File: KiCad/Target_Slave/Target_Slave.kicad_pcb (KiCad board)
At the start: 2 copper layers, 76.2 x 50.8 mm, 44 parts, among them J1 ICSP, J2 I2C, J3 I2C, SW1 I2C Address, U1 PIC16F1788-IP, U2 TSSP4038, U3 TSOP53456

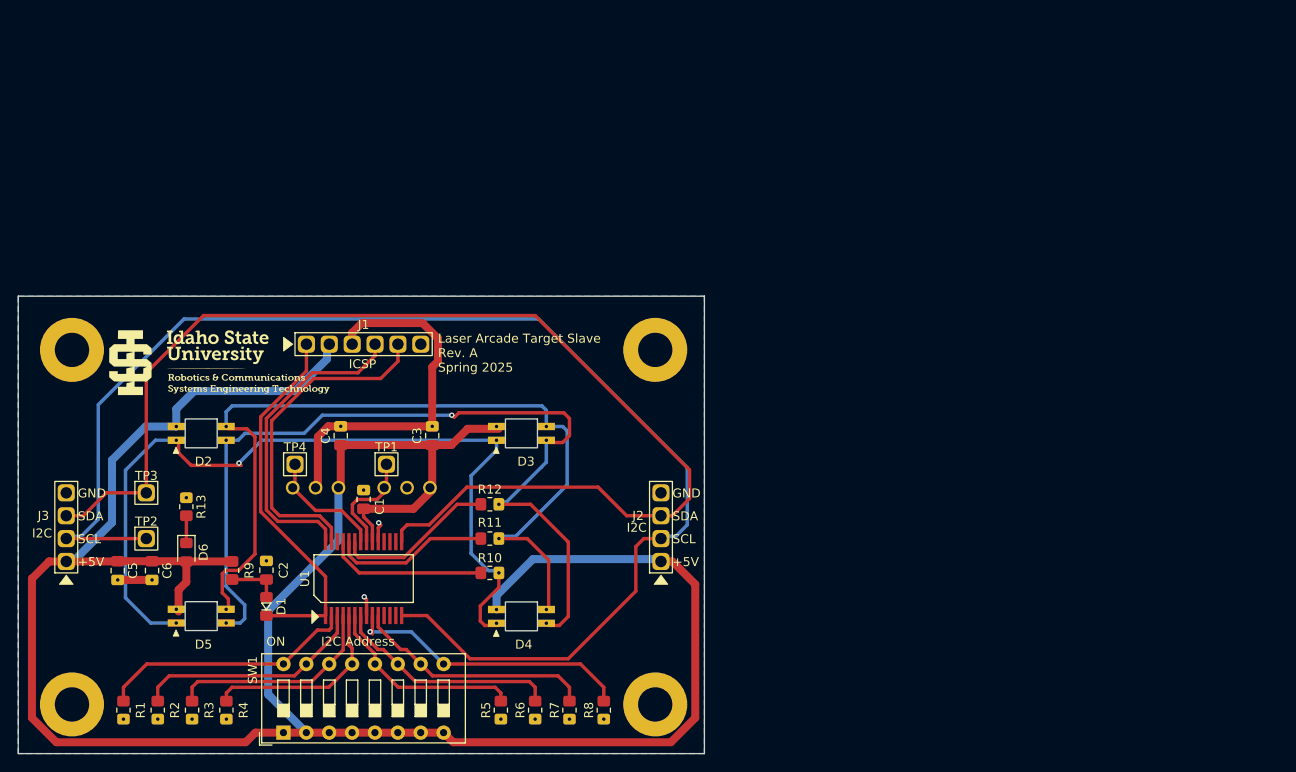
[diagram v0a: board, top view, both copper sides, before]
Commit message: Rev B Target Slave PCB design
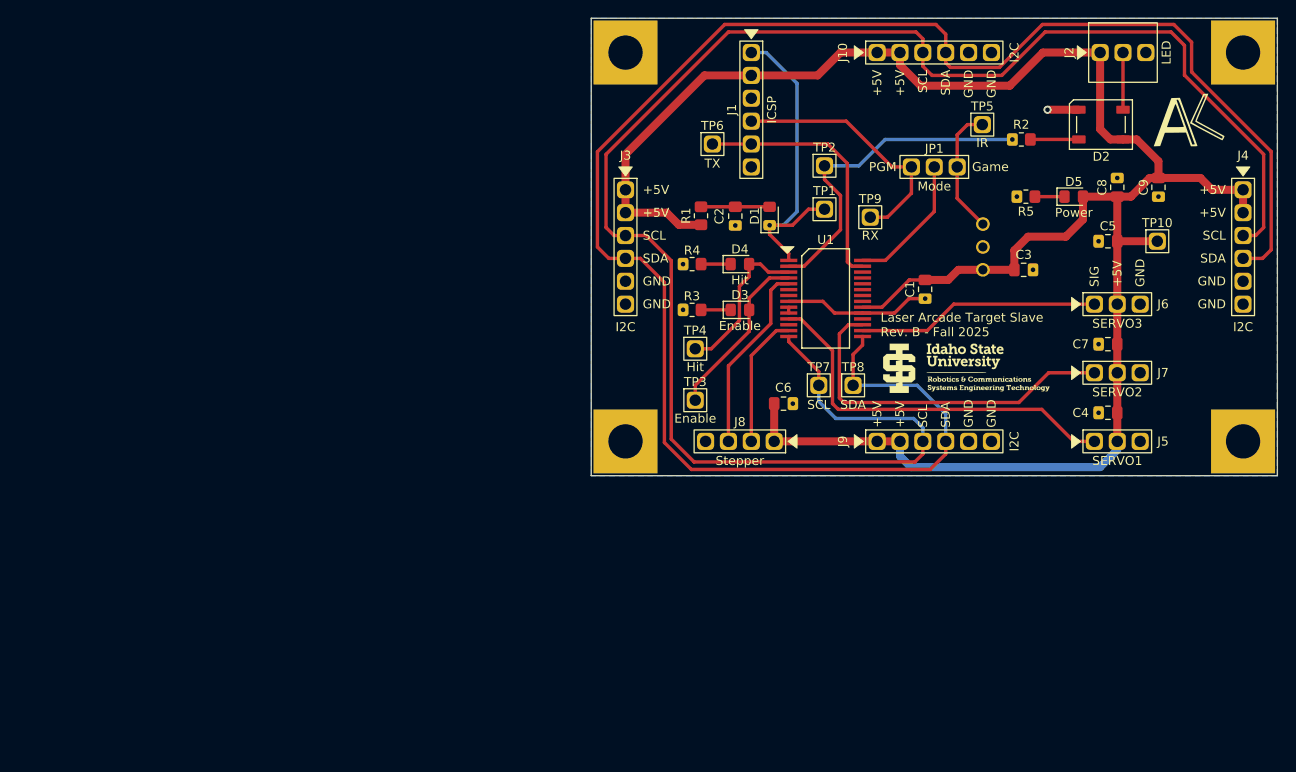
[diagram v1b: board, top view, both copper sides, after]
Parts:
- removed ? (x3): , 
- removed D6: LED, LED_SMD:LED_0805_2012Metric_Pad1.15x1.40mm_HandSolder
- removed the G*** at (135.4, 83.2)
- removed the G*** at (132.0, 118.1)
- removed the G*** at (121.2, 112.8)
- removed R10, R12: 90Ω, Resistor_SMD:R_0805_2012Metric_Pad1.20x1.40mm_HandSolder
- removed R11: 150Ω, Resistor_SMD:R_0805_2012Metric_Pad1.20x1.40mm_HandSolder
- removed R13: 4.7kΩ, Resistor_SMD:R_0805_2012Metric_Pad1.20x1.40mm_HandSolder
- removed R6, R7, R8: 330Ω, Resistor_SMD:R_0805_2012Metric_Pad1.20x1.40mm_HandSolder
- removed R9: 10kΩ, Resistor_SMD:R_0805_2012Metric_Pad1.20x1.40mm_HandSolder
- removed the REF** at (183.6, 81.9)
- removed SW1: I2C Address, 0_AKeller_Footprints:SW_DIP_SPSTx08_Slide_9.78x22.5mm_W7.62mm_P2.54mm
- removed U3: TSOP53456, 0_AKeller_Footprints:IR Receiver
- added C7: 1µF, Capacitor_SMD:C_0805_2012Metric_Pad1.18x1.45mm_HandSolder, F.Cu at (233.9, 81.3)
- added C8: 22uF, Capacitor_SMD:C_0805_2012Metric_Pad1.18x1.45mm_HandSolder, F.Cu at (234.9, 63.9)
- added C9: 0.1uF, Capacitor_SMD:C_0805_2012Metric_Pad1.18x1.45mm_HandSolder, F.Cu at (239.5, 63.9)
- added G***: LOGO, 2025 Logos:AKeller_Logo_0-23x0-31, F.Cu at (243.0, 56.4)
- added G***: LOGO, 2025 Logos:RCET Stacked 0-25x0_76, F.Cu at (218.3, 83.8)
- added J10: I2C, 0_AKeller_Footprints:1x6_100mil_Header, F.Cu at (214.6, 48.9)
- added J4: I2C, 0_AKeller_Footprints:1x6_100mil_Header, F.Cu at (248.9, 70.5)
- added J5: SERVO1, 0_AKeller_Footprints:1x3_100mil_Header, F.Cu at (234.9, 92.1)
- added J6: SERVO3, 0_AKeller_Footprints:1x3_100mil_Header, F.Cu at (234.9, 76.8)
- added J7: SERVO2, 0_AKeller_Footprints:1x3_100mil_Header, F.Cu at (234.9, 84.5)
- added J8: Stepper, 0_AKeller_Footprints:1x4_100mil_Header, F.Cu at (193.0, 92.1)
- added J9: I2C, 0_AKeller_Footprints:1x6_100mil_Header, F.Cu at (214.6, 92.1)
- added JP1: Mode, 0_AKeller_Footprints:1x3_100mil_Jumper, F.Cu at (214.6, 61.6)
- added REF**: M3 Mounting, 0_AKeller_Footprints:M3 Mounting, F.Cu at (180.3, 92.1)
- added REF**: M3 Mounting, 0_AKeller_Footprints:M3 Mounting, F.Cu at (248.9, 92.1)
- added REF**: M3 Mounting, 0_AKeller_Footprints:M3 Mounting, F.Cu at (180.3, 48.9)
- added REF**: M3 Mounting, 0_AKeller_Footprints:M3 Mounting, F.Cu at (248.9, 48.9)
- added TP10: PWR, 0_AKeller_Footprints:1x1_100mil_Header, F.Cu at (239.4, 69.8)
- added TP5: IR, 0_AKeller_Footprints:1x1_100mil_Header, F.Cu at (220.0, 56.9)
- added TP6: TX, 0_AKeller_Footprints:1x1_100mil_Header, F.Cu at (190.0, 59.1)
- added TP7: SCL, 0_AKeller_Footprints:1x1_100mil_Header, F.Cu at (201.8, 85.9)
- added TP8: SDA, 0_AKeller_Footprints:1x1_100mil_Header, F.Cu at (205.6, 85.9)
- added TP9: RX, 0_AKeller_Footprints:1x1_100mil_Header, F.Cu at (207.5, 67.2)
- C4: value 1uF -> 1µF
- C5: value 22uF -> 1µF
- C6: value 0.1uF -> 1µF
- D1: footprint 0_AKeller_Footprints:Diode_0805 -> Diode_SMD:D_0805_2012Metric_Pad1.15x1.40mm_HandSolder
- D2: value IN-P32TRRRGB -> WS2812B; footprint 0_AKeller_Footprints:IN-P32TRRRGB -> LED_SMD:LED_WS2812B_PLCC4_5.0x5.0mm_P3.2mm; moved to F.Cu
- D3: value IN-P32TRRRGB -> Enable; footprint 0_AKeller_Footprints:IN-P32TRRRGB -> LED_SMD:LED_0805_2012Metric_Pad1.15x1.40mm_HandSolder; moved to F.Cu
- D4: value IN-P32TRRRGB -> Hit; footprint 0_AKeller_Footprints:IN-P32TRRRGB -> LED_SMD:LED_0805_2012Metric_Pad1.15x1.40mm_HandSolder; moved to F.Cu
- D5: value IN-P32TRRRGB -> Power; footprint 0_AKeller_Footprints:IN-P32TRRRGB -> LED_SMD:LED_0805_2012Metric_Pad1.15x1.40mm_HandSolder; moved to F.Cu
- J2: value I2C -> LED; footprint 0_AKeller_Footprints:1x4_100mil_Header -> 0_AKeller_Footprints:1x3_100mil_Header_Locking
- J3: footprint 0_AKeller_Footprints:1x4_100mil_Header -> 0_AKeller_Footprints:1x6_100mil_Header
- R1: value 330Ω -> 10kΩ
- R2: value 330Ω -> 470Ω
- R3, R4, R5: value 330Ω -> 4.7kΩ
- TP1: value ~ -> MCLR
- TP2: value ~ -> RGB_IN
- TP3: value ~ -> Enable
- TP4: value ~ -> Hit
- moved C5 115.9 mm to (233.9, 69.8), turned to 0 degrees
- moved R2 114.9 mm to (224.3, 58.5), turned to 0 degrees
- moved D5 107.5 mm to (230.1, 64.9), turned to 0 degrees
- moved D2 105.6 mm to (233.1, 56.9)
- moved TP2 85.9 mm to (202.4, 61.5)
- moved C4 85.2 mm to (233.9, 88.9), turned to 0 degrees
- moved R1 84.4 mm to (188.7, 67.0)
- moved R5 81.6 mm to (224.8, 64.9), turned to 180 degrees
- moved J2 73.6 mm to (235.6, 48.9), turned to 0 degrees
- moved C6 72.5 mm to (197.9, 87.9), turned to 180 degrees
- moved R4 71.6 mm to (187.7, 72.4), turned to 180 degrees
- moved R3 71.1 mm to (187.7, 77.5), turned to 180 degrees
- moved D1 70.7 mm to (196.3, 67.0)
- moved J3 69.5 mm to (180.3, 70.5), turned to -90 degrees
- moved U2 69.3 mm to (220.0, 70.5), turned to -90 degrees
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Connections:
- net RB6 renamed TX
- C4 pad 1: +5V -> GND
- C4 pad 2: GND -> +5V
- C5 pad 1: +5V -> GND
- C5 pad 2: GND -> +5V
- C6 pad 1: +5V -> GND
- C6 pad 2: GND -> +5V
- D1 pad 1: Net-(D1-K) -> /MCLR
- D2 pad 1: Net-(D2-BK) -> +5V
- D2 pad 2: Net-(D2-GK) -> Net-(D2-DOUT)
- D2 pad 3: Net-(D2-RK) -> GND
- D2 pad 4: +5V -> Net-(D2-DIN)
- D3 pad 1: Net-(D2-BK) -> Net-(D3-K)
- D3 pad 2: Net-(D2-GK) -> Net-(D3-A)
- D4 pad 1: Net-(D2-BK) -> Net-(D4-K)
- D4 pad 2: Net-(D2-GK) -> Net-(D4-A)
- D5 pad 1: Net-(D2-BK) -> Net-(D5-K)
- D5 pad 2: Net-(D2-GK) -> +5V
- J1 pad 1: Net-(D1-K) -> /MCLR
- J1 pad 4: RB7 -> RX
- J2 pad 2: Net-(U1-RC3/SCK/SCL) -> Net-(D2-DOUT)
- J2 pad 3: Net-(U1-RC4/SDI/SDA) -> GND
- J3 pad 2: Net-(U1-RC3/SCK/SCL) -> +5V
- J3 pad 3: Net-(U1-RC4/SDI/SDA) -> /SCL
- J3 pad 4: GND -> /SDA
- R1 pad 1: GND -> +5V
- R1 pad 2: /RA0 -> Net-(D1-A)
- R2 pad 1: GND -> Net-(U1-ULPWU/C12IN0-/AN0/RA0)
- R2 pad 2: /RA1 -> Net-(D2-DIN)
- R3 pad 1: GND -> Net-(D3-K)
- R3 pad 2: /RA2 -> GND
- R4 pad 1: GND -> Net-(D4-K)
- R4 pad 2: /RA3 -> GND
- R5 pad 1: GND -> Net-(D5-K)
- R5 pad 2: /RA4 -> GND
- TP1 pad 1: Net-(U1-INT/AN12/RB0) -> /MCLR
- TP2 pad 1: Net-(U1-RC3/SCK/SCL) -> Net-(U1-ULPWU/C12IN0-/AN0/RA0)
- TP3 pad 1: Net-(U1-RC4/SDI/SDA) -> Net-(D3-A)
- TP4 pad 1: Net-(U1-P1C/AN10/RB1) -> Net-(D4-A)
- U1 pad 1: Net-(D1-K) -> /MCLR
- U1 pad 10: /RA6 -> Net-(U1-CLKIN/OSC1/RA7)
- U1 pad 11: unconnected-(U1-RC0/T1OSO/T1CK1-Pad11) -> SERVO1
- U1 pad 13: unconnected-(U1-RC2/P1A/CCP1-Pad13) -> STEP
- U1 pad 14: Net-(U1-RC3/SCK/SCL) -> /SCL
- U1 pad 15: Net-(U1-RC4/SDI/SDA) -> /SDA
- U1 pad 16: unconnected-(U1-RC5/SDO-Pad16) -> SERVO3
- U1 pad 17: unconnected-(U1-RC6/TX/CK-Pad17) -> SERVO2
- U1 pad 2: /RA0 -> Net-(U1-ULPWU/C12IN0-/AN0/RA0)
- U1 pad 21: Net-(U1-INT/AN12/RB0) -> unconnected-(U1-INT/AN12/RB0-Pad21)
- U1 pad 22: Net-(U1-P1C/AN10/RB1) -> unconnected-(U1-P1C/AN10/RB1-Pad22)
- U1 pad 23: Net-(U1-P1B/AN8/RB2) -> unconnected-(U1-P1B/AN8/RB2-Pad23)
- U1 pad 24: Net-(U1-PGM/C12IN2-/AN8/RB3) -> unconnected-(U1-PGM/C12IN2-/AN8/RB3-Pad24)
- U1 pad 25: Net-(U1-P1D/AN11/RB4) -> unconnected-(U1-P1D/AN11/RB4-Pad25)
- U1 pad 28: RB7 -> Net-(JP1-C)
- U1 pad 3: /RA1 -> Net-(D4-A)
- U1 pad 4: /RA2 -> Net-(D3-A)
- U1 pad 5: /RA3 -> DIR
- U1 pad 6: /RA4 -> unconnected-(U1-T0CKI/C1OUT/RA4-Pad6)
- U1 pad 7: /RA5 -> unconnected-(U1-~{SS}/C2OUT/AN4/RA5-Pad7)
- U1 pad 9: /RA7 -> Net-(U1-CLKIN/OSC1/RA7)
- U2 pad 1: Net-(U1-INT/AN12/RB0) -> Net-(JP1-A)
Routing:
- net /SDA: track 0.00 -> 201.2 mm
- net /SCL: track 0.00 -> 193.1 mm
- net Net-(U1-RC3/SCK/SCL): track 151.6 -> 0.00 mm
- net Net-(U1-RC4/SDI/SDA): track 133.8 -> 0.00 mm
- net Net-(D2-GK): track 97.1 -> 0.00 mm, vias 1 -> 0
- net Net-(D2-RK): track 95.8 -> 0.00 mm
- net Net-(D2-BK): track 92.1 -> 0.00 mm, vias 1 -> 0
- net +5V: track 280.4 -> 226.8 mm
- net SERVO1: track 0.00 -> 43.0 mm
- net Net-(D1-K): track 41.8 -> 0.00 mm
- net SERVO2: track 0.00 -> 40.0 mm
- net Net-(U1-ULPWU/C12IN0-/AN0/RA0): track 0.00 -> 37.3 mm
- net /MCLR: track 0.00 -> 36.0 mm
- net RB7: track 35.2 -> 0.00 mm
- net /RA7: track 31.8 -> 0.00 mm, vias 1 -> 0
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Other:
- board text added: "Game"
- board text added: "Laser Arcade Target Slave Rev. B - Fall 2025"
- board text added: "PGM"
- board text added: "SIG"
- board text removed: "D2"
- board text removed: "D3"
- board text removed: "D4"
- board text removed: "D5"
- board text removed: "I2C"
- board text removed: "ICSP"
- board text removed: "Laser Arcade Target Slave Rev. A Spring 2025"
